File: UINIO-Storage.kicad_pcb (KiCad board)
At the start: 2 copper layers, 60 x 42 mm, 51 parts, among them J1 Conn_01x04_Pin, J2 Conn_01x04_Pin, J3 Conn_01x06_Pin, J4 Conn_01x08_Pin, J5 Conn_01x06_Pin, U1 I2C-24-EEPROM-SOIC8, U2 I2C-24-EEPROM-TSSOP8, U3 SPI-25-Flash-SOIC8, U4 ME6211, U5 SPI-25-Flash-WSON8

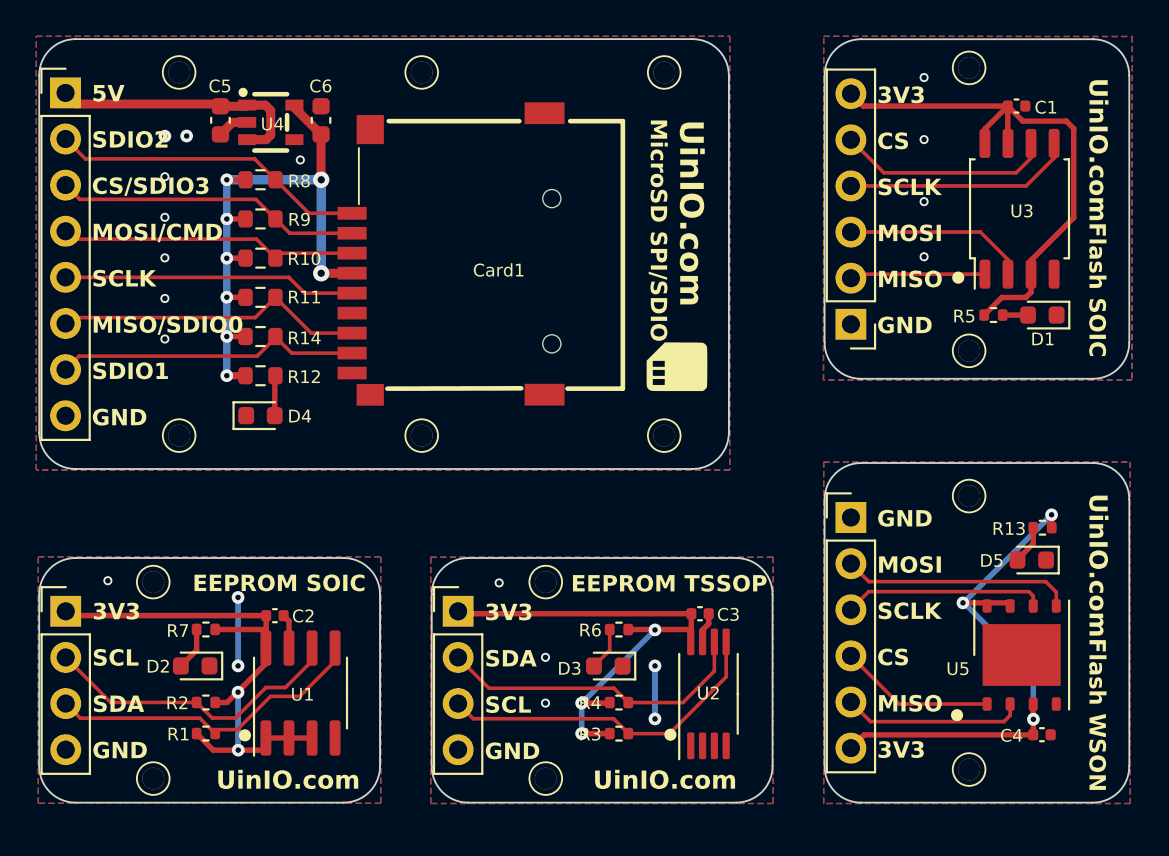
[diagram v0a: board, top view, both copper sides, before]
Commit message: Complete PCB wiring.
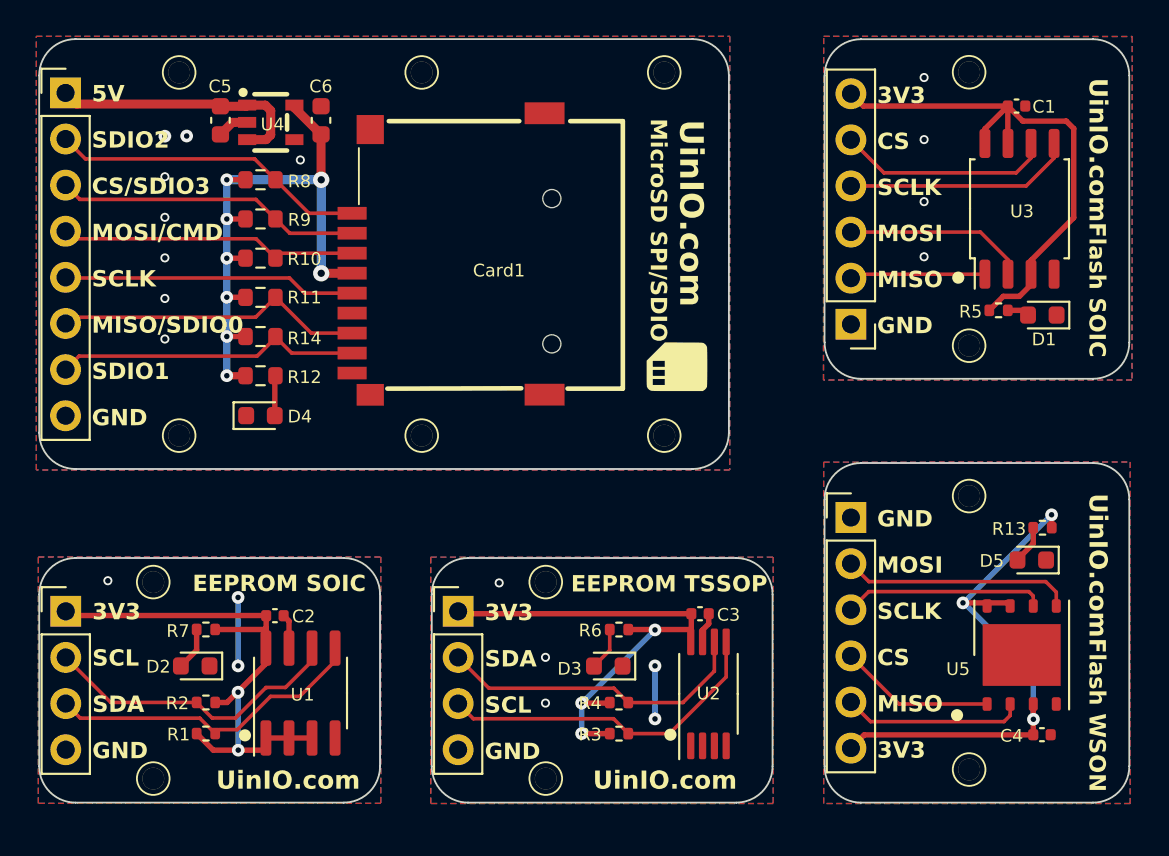
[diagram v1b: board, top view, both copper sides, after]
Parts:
- removed the HOLE** at (172.8, 100.3)
- removed the HOLE** at (172.8, 84.8)
- added HOLE**: Hole-1mm, Uinio:Hole-1mm, F.Cu at (172.8, 85.0)
- added HOLE**: Hole-1mm, Uinio:Hole-1mm, F.Cu at (172.8, 100.0)
- moved R5 0.38 mm to (174.4, 98.1)
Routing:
- net /Flash-SOIC8-3.3V: track 30.8 -> 29.6 mm
- net Net-(D1-A): track 1.39 -> 0.85 mm
